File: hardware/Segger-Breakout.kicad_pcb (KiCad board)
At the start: 2 copper layers, 116.8 x 111.8 mm, 12 parts, among them J1 ESP32Pro Breakout2, J2 ESP32Pro Breakout1, J4 JTag Segger Connector, J5 Rpi Pico Breakout1, J6 Rpi Pico Breakout2, J7 Segger 5V Out, J8 Segger Breakout, P1 JTAG SWD Connector, U1 ProS3, U2 Rpi Pico

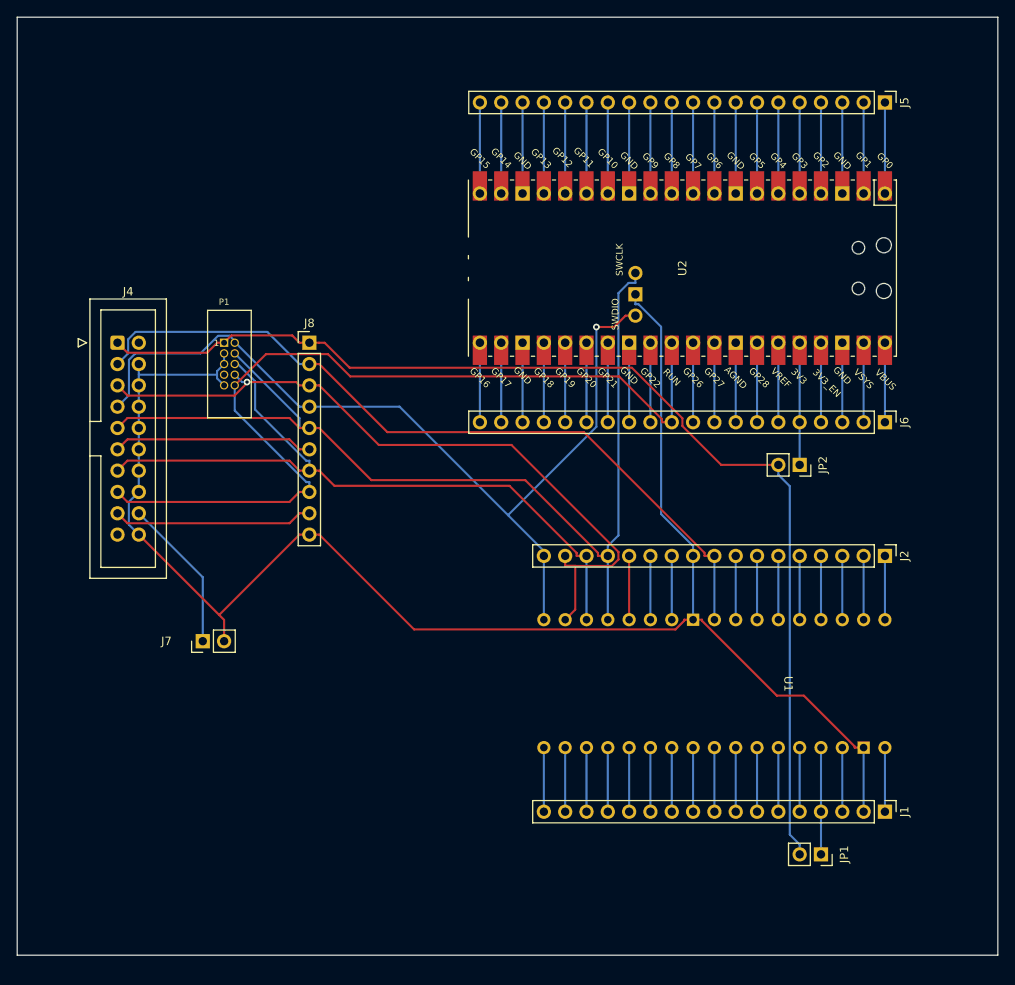
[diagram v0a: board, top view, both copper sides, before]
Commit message: pcb updates
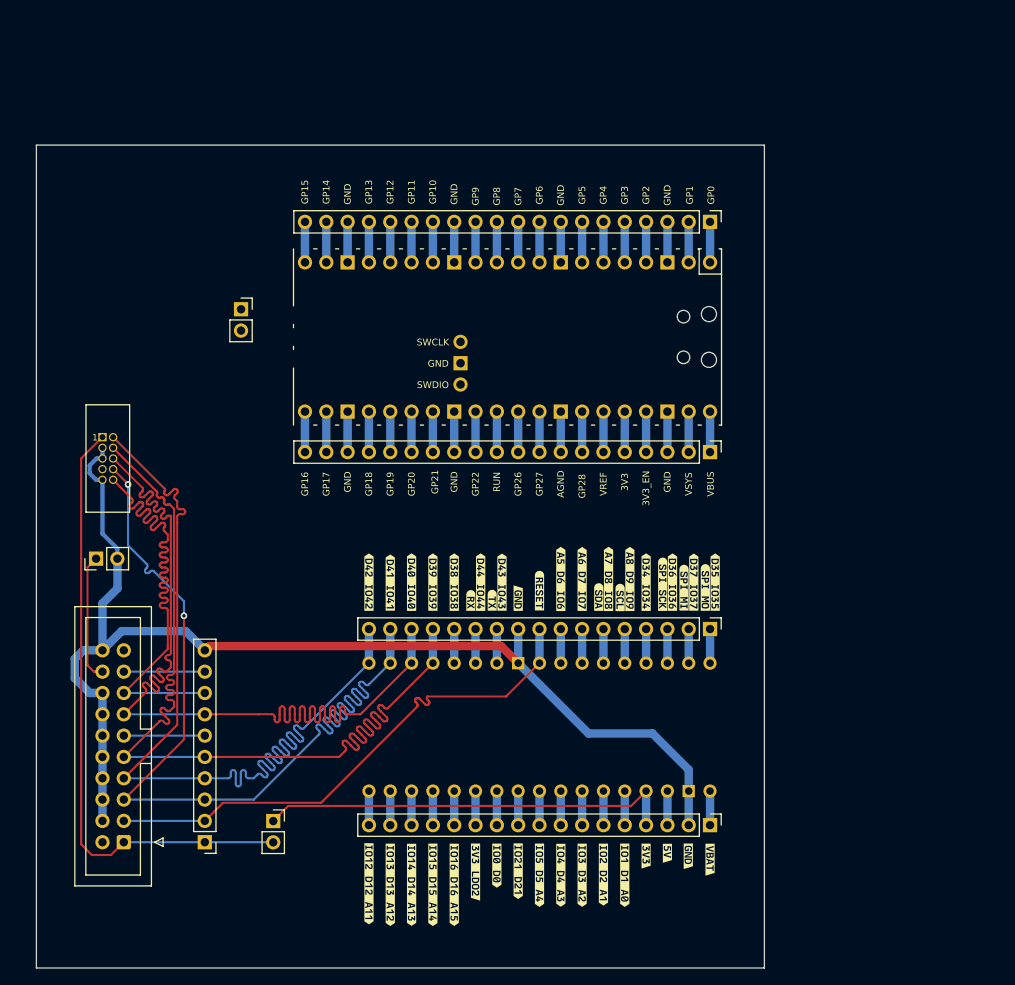
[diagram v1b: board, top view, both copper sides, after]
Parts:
- added kibuzzard-655FC45E: G***, kibuzzard-655FC45E, F.Cu at (146.1, 132.7)
- added kibuzzard-655FC469: G***, kibuzzard-655FC469, F.Cu at (143.5, 132.6)
- added kibuzzard-655FC471: G***, kibuzzard-655FC471, F.Cu at (141.0, 132.7)
- added kibuzzard-655FC478: G***, kibuzzard-655FC478, F.Cu at (138.4, 132.7)
- added kibuzzard-655FC4B1: G***, kibuzzard-655FC4B1, F.Cu at (135.9, 132.7)
- added kibuzzard-655FC52C: G***, kibuzzard-655FC52C, F.Cu at (133.3, 132.2)
- added kibuzzard-655FC56D: G***, kibuzzard-655FC56D, F.Cu at (130.8, 131.6)
- added kibuzzard-655FC607: G***, kibuzzard-655FC607, F.Cu at (128.3, 132.3)
- added kibuzzard-655FC60E: G***, kibuzzard-655FC60E, F.Cu at (148.6, 130.4)
- added kibuzzard-655FC616: G***, kibuzzard-655FC616, F.Cu at (151.1, 130.1)
- added kibuzzard-655FC61C: G***, kibuzzard-655FC61C, F.Cu at (153.6, 130.5)
- added kibuzzard-655FC635: G***, kibuzzard-655FC635, F.Cu at (156.2, 130.9)
- added kibuzzard-655FC6B9: G***, kibuzzard-655FC6B9, F.Cu at (125.7, 133.9)
- added kibuzzard-655FC710: G***, kibuzzard-655FC710, F.Cu at (123.2, 133.9)
- added kibuzzard-655FC738: G***, kibuzzard-655FC738, F.Cu at (120.7, 133.9)
- added kibuzzard-655FC7B2: G***, kibuzzard-655FC7B2, F.Cu at (118.1, 133.9)
- added kibuzzard-655FC7D9: G***, kibuzzard-655FC7D9, F.Cu at (115.6, 133.7)
- added kibuzzard-655FC940: G***, kibuzzard-655FC940, F.Cu at (156.8, 97.8)
- added kibuzzard-655FC954: G***, kibuzzard-655FC954, F.Cu at (154.3, 97.8)
- added kibuzzard-655FC9E7: G***, kibuzzard-655FC9E7, F.Cu at (151.7, 97.8)
- added kibuzzard-655FCA04: G***, kibuzzard-655FCA04, F.Cu at (148.6, 97.8)
- added kibuzzard-655FCA38: G***, kibuzzard-655FCA38, F.Cu at (146.7, 97.4)
- added kibuzzard-655FCA61: G***, kibuzzard-655FCA61, F.Cu at (144.1, 97.4)
- added kibuzzard-655FCA7F: G***, kibuzzard-655FCA7F, F.Cu at (141.0, 97.4)
- added kibuzzard-655FCAAA: G***, kibuzzard-655FCAAA, F.Cu at (138.4, 97.4)
- added kibuzzard-655FCAFA: G***, kibuzzard-655FCAFA, F.Cu at (155.7, 98.4)
- added kibuzzard-655FCB2A: G***, kibuzzard-655FCB2A, F.Cu at (153.1, 98.5)
- added kibuzzard-655FCBAC: G***, kibuzzard-655FCBAC, F.Cu at (150.6, 98.0)
- added kibuzzard-655FCC1E: G***, kibuzzard-655FCC1E, F.Cu at (131.4, 97.8)
- added kibuzzard-655FCC41: G***, kibuzzard-655FCC41, F.Cu at (133.3, 99.7)
- added kibuzzard-655FCC6B: G***, kibuzzard-655FCC6B, F.Cu at (135.9, 98.8)
- added kibuzzard-655FCC8E: G***, kibuzzard-655FCC8E, F.Cu at (128.9, 97.8)
- added kibuzzard-655FCCA3: G***, kibuzzard-655FCCA3, F.Cu at (145.5, 99.6)
- added kibuzzard-655FCCAF: G***, kibuzzard-655FCCAF, F.Cu at (143.0, 99.6)
- added kibuzzard-655FCD75: G***, kibuzzard-655FCD75, F.Cu at (125.7, 97.8)
- added kibuzzard-655FCDA8: G***, kibuzzard-655FCDA8, F.Cu at (123.2, 97.8)
- added kibuzzard-655FCDCF: G***, kibuzzard-655FCDCF, F.Cu at (120.7, 97.8)
- added kibuzzard-655FCDDC: G***, kibuzzard-655FCDDC, F.Cu at (118.1, 97.8)
- added kibuzzard-655FCE13: G***, kibuzzard-655FCE13, F.Cu at (115.6, 97.8)
- added kibuzzard-655FCE50: G***, kibuzzard-655FCE50, F.Cu at (130.3, 99.9)
- added kibuzzard-655FCE5C: G***, kibuzzard-655FCE5C, F.Cu at (127.7, 100.0)
- JP1, JP2: value VTref Segger Input -> VTref Input
- moved JP2 69.1 mm to (100.3, 65.3), turned to 0 degrees
- moved JP1 65.4 mm to (104.2, 126.3), turned to 0 degrees
- moved J8 60.8 mm to (96.0, 128.8), turned to 180 degrees
- moved J4 59.5 mm to (86.4, 128.8), turned to 180 degrees
- moved J5 25.2 mm to (156.2, 54.9)
- moved J2 22.6 mm to (156.2, 103.4)
- moved U2 22.4 mm to (132.1, 68.6)
- moved U1 21.5 mm to (135.9, 115.1)
- moved J6 21.1 mm to (156.2, 82.3)
- moved J1 20.9 mm to (156.2, 126.7)
- moved P1 18.3 mm to (84.5, 83.1)
- moved J7 16.1 mm to (83.1, 95.0)
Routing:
- net /JTAG.VTRef: track 134.5 -> 73.6 mm
- net GND: track 194.0 -> 141.7 mm
- net /JTAG.RESET: track 107.1 -> 63.9 mm
- net Net-(J1-Pin_4): track 12.7 -> 50.0 mm
- net /JTAG.~{nTRST}: track 92.6 -> 63.7 mm
- net /JTAG.TDO: track 85.7 -> 113.0 mm
- net /JTAG.TDI: track 86.8 -> 110.2 mm, vias 1 -> 2
- net /JTAG.RTCK: track 23.8 -> 9.65 mm
- net /JTAG.DBGRQ: track 23.8 -> 9.65 mm
- net Net-(J6-Pin_5): track 14.6 -> 4.83 mm
- net /JTAG.TCK: track 122.3 -> 113.2 mm
- net Net-(J5-Pin_9): track 10.8 -> 4.83 mm
- net Net-(J5-Pin_8): track 10.8 -> 4.83 mm
- net Net-(J5-Pin_7): track 10.8 -> 4.83 mm
- net Net-(J5-Pin_6): track 10.8 -> 4.83 mm
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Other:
- board size 116.8 x 111.8 mm -> 86.7 x 98 mm
